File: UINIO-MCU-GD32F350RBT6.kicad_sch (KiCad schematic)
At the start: 1 part

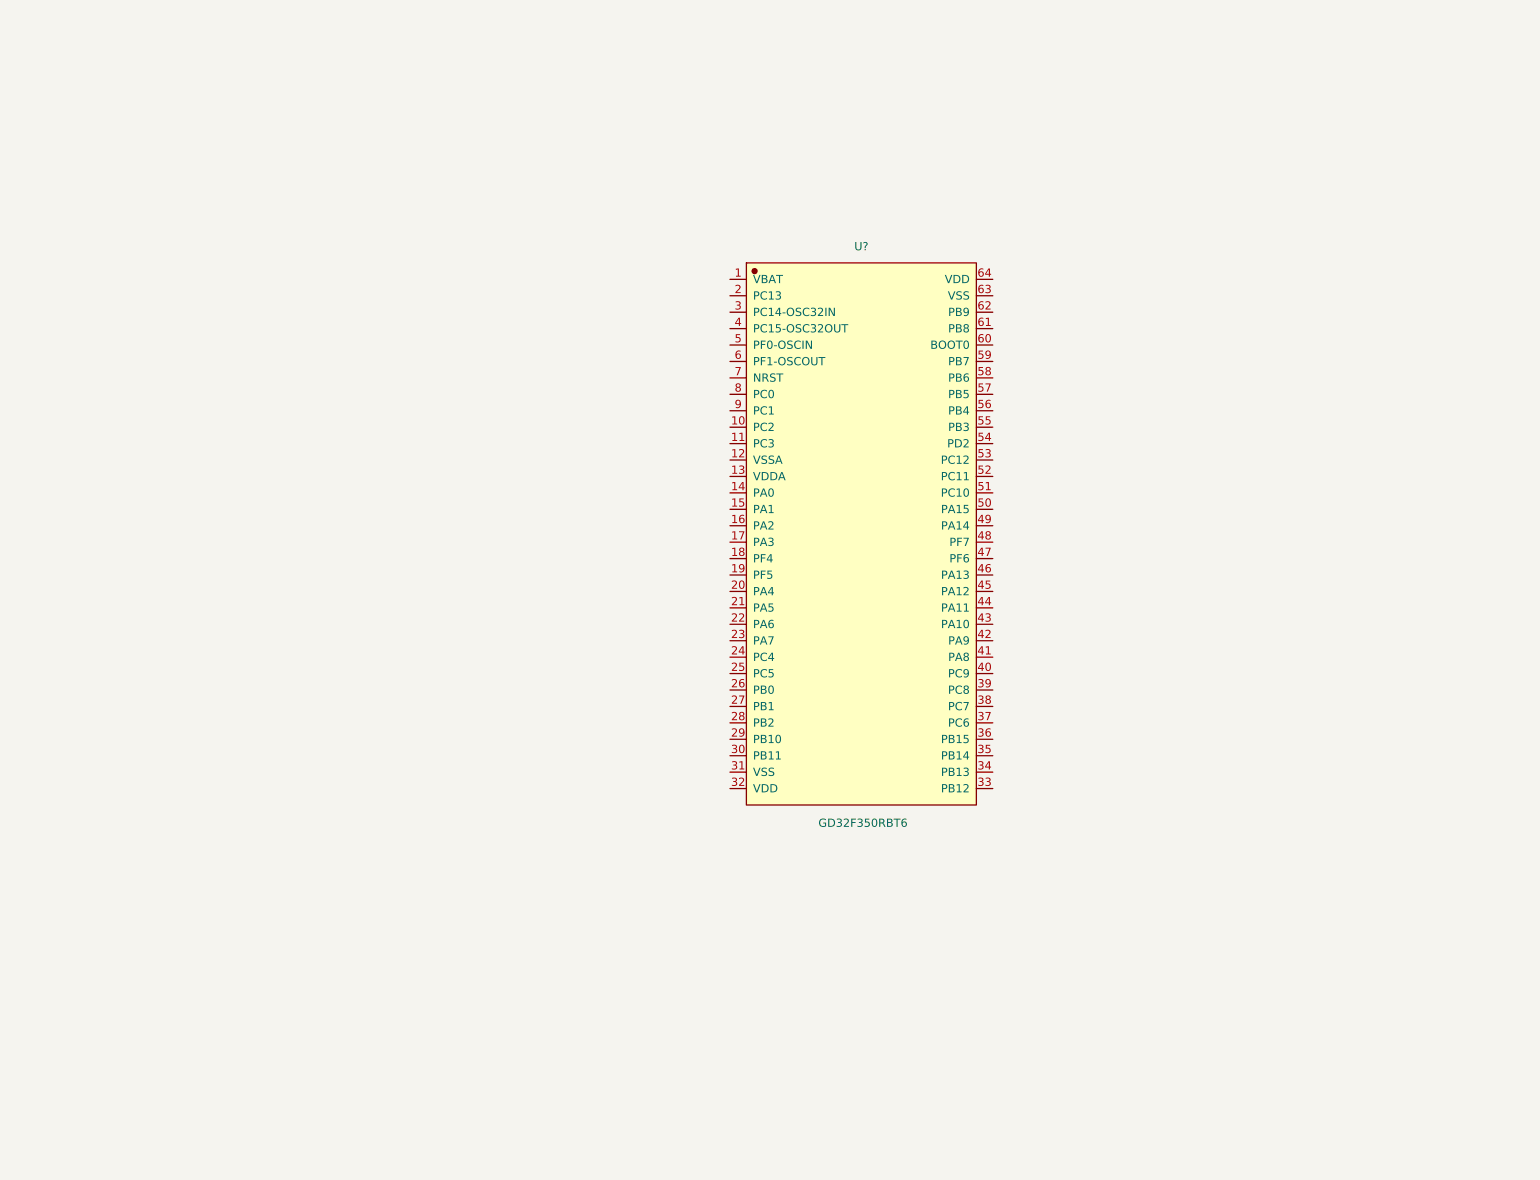
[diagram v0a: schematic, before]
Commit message: Initializing the project
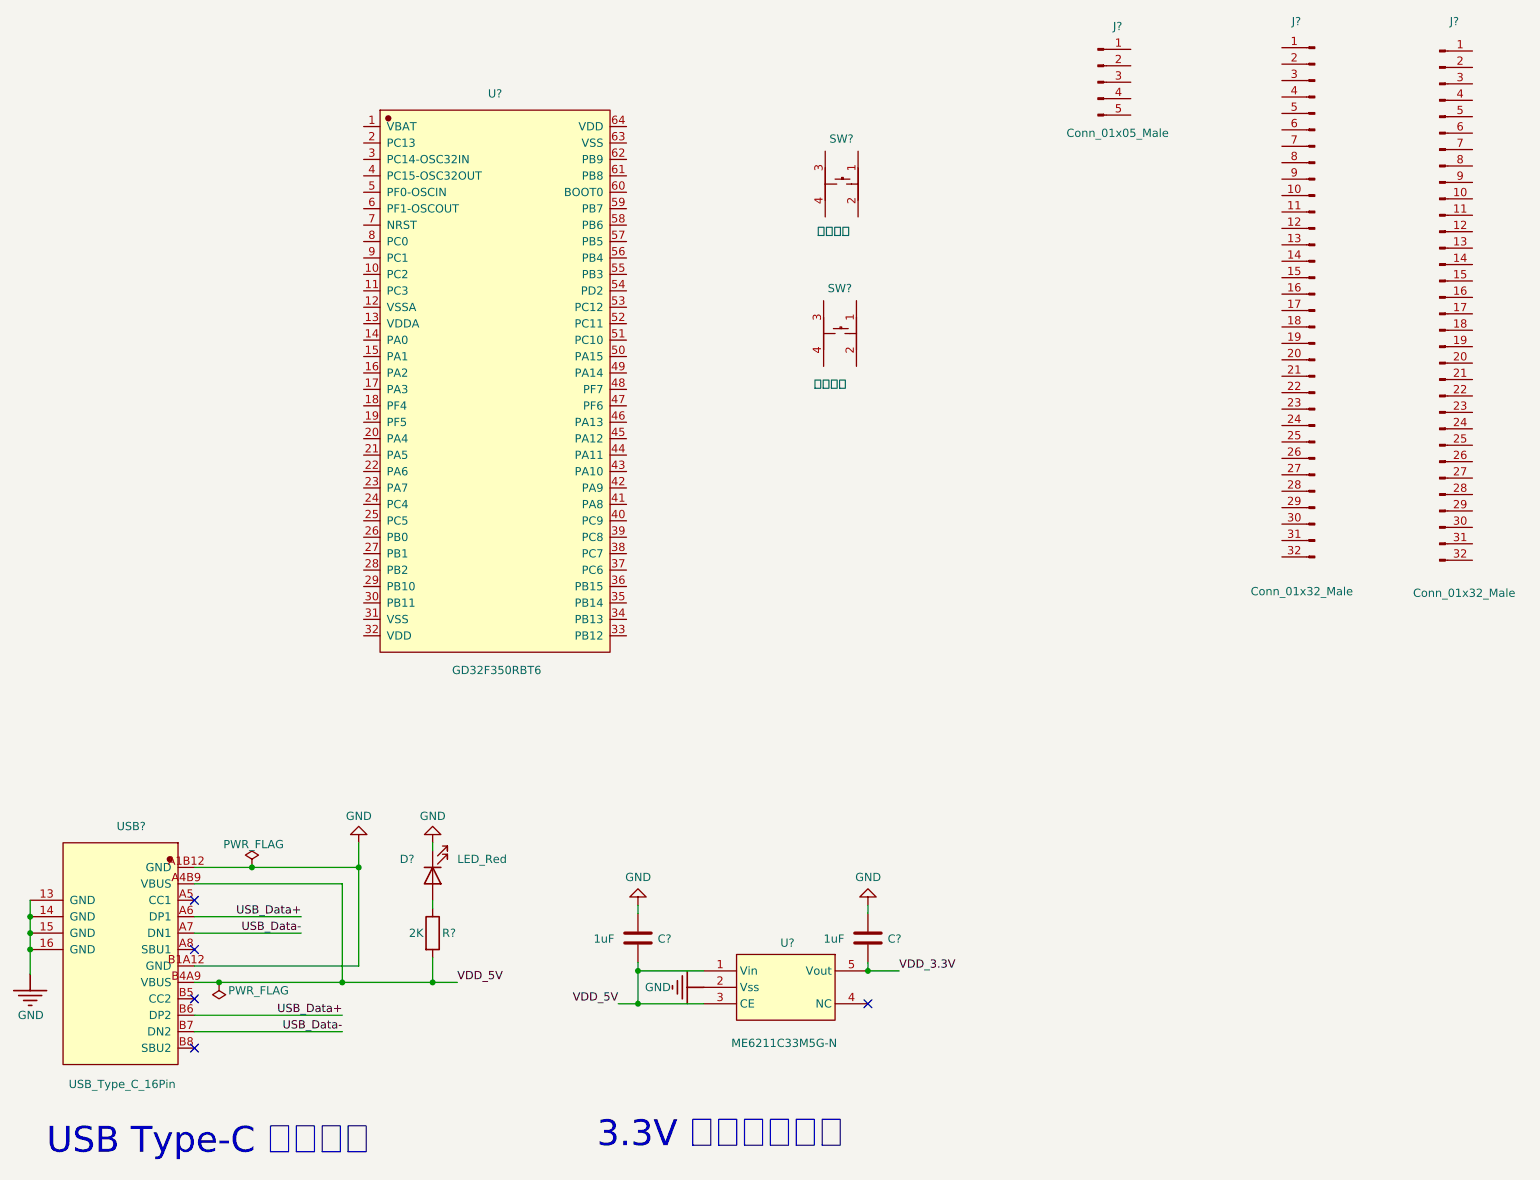
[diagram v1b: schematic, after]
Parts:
- added C? (x2): 1uF, Capacitor_SMD:C_0402_1005Metric, symbol Device:C
- added D?: LED_Red, LED_SMD:LED_0603_1608Metric, symbol Device:LED
- added J? (x2): Conn_01x32_Male, symbol Connector:Conn_01x32_Male
- added J?: Conn_01x05_Male, symbol Connector:Conn_01x05_Male
- added R?: 2K, Resistor_SMD:R_0402_1005Metric, symbol Device:R
- added SW?: 下载按键, Uinio:KEY-SMD_4P-L4.2-W3.4-P2.15-LS4.7, symbol Uinio:Key_YTS_A016S_1
- added SW?: 复位按键, Uinio:KEY-SMD_4P-L4.2-W3.4-P2.15-LS4.7, symbol Uinio:Key_YTS_A016S_1
- added U?: ME6211C33M5G-N, Uinio:SOT-23-5_L3.0-W1.7-P0.95-LS2.8-BR, symbol Uinio:ME6211
- added USB?: USB_Type_C_16Pin, Uinio:USB-C-SMD_TYPEC-304J-BCP16, symbol Uinio:USB_Type_C_16Pin
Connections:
- new net: D?.2 (A), R?.1
- new net GND: C?.1, C?.1, D?.1 (K), U?.2 (Vss), USB?.13 (GND), USB?.14 (GND), USB?.15 (GND), USB?.16 (GND), USB?.A1B12 (GND), USB?.B1A12 (GND)
- new net USB_Data+: USB?.A6 (DP1), USB?.B6 (DP2)
- new net USB_Data-: USB?.A7 (DN1), USB?.B7 (DN2)
- new net VDD_3.3V: C?.2, U?.5 (Vout)
- new net VDD_5V: C?.2, R?.2, U?.1 (Vin), U?.3 (CE), USB?.A4B9 (VBUS), USB?.B4A9 (VBUS)
- no-connect marks 0 -> 5
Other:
- note added: "3.3V 线性稳压电路"
- note added: "USB Type-C 接口电路"
- moved on the sheet: U?
